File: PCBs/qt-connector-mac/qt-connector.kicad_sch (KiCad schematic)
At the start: 4 parts, among them K1 Quicktake, K2 Modem port, K3 Printer port, K4 ImageWriter

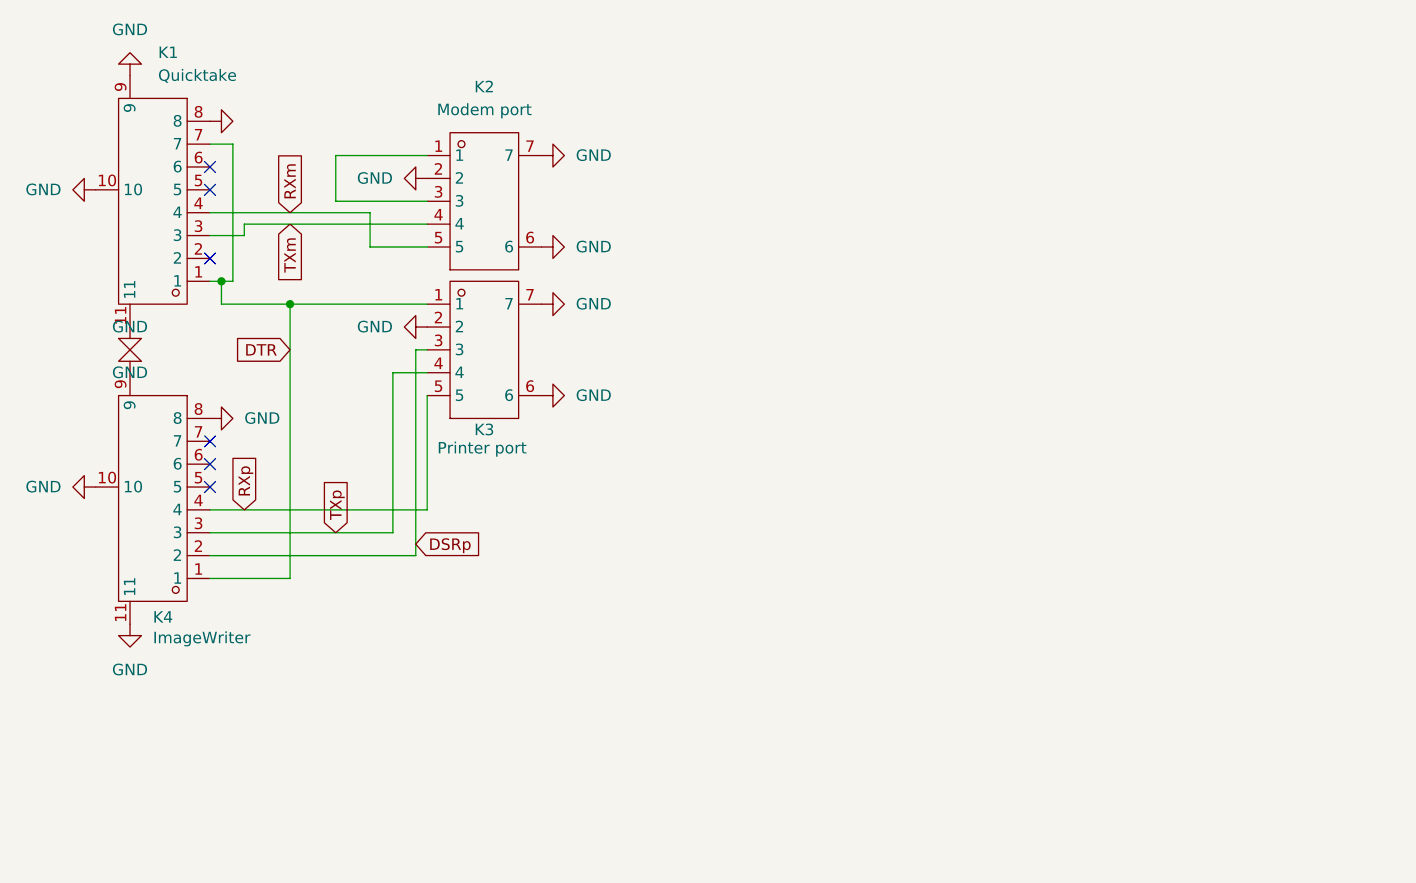
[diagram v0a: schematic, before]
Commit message: Update to new lib
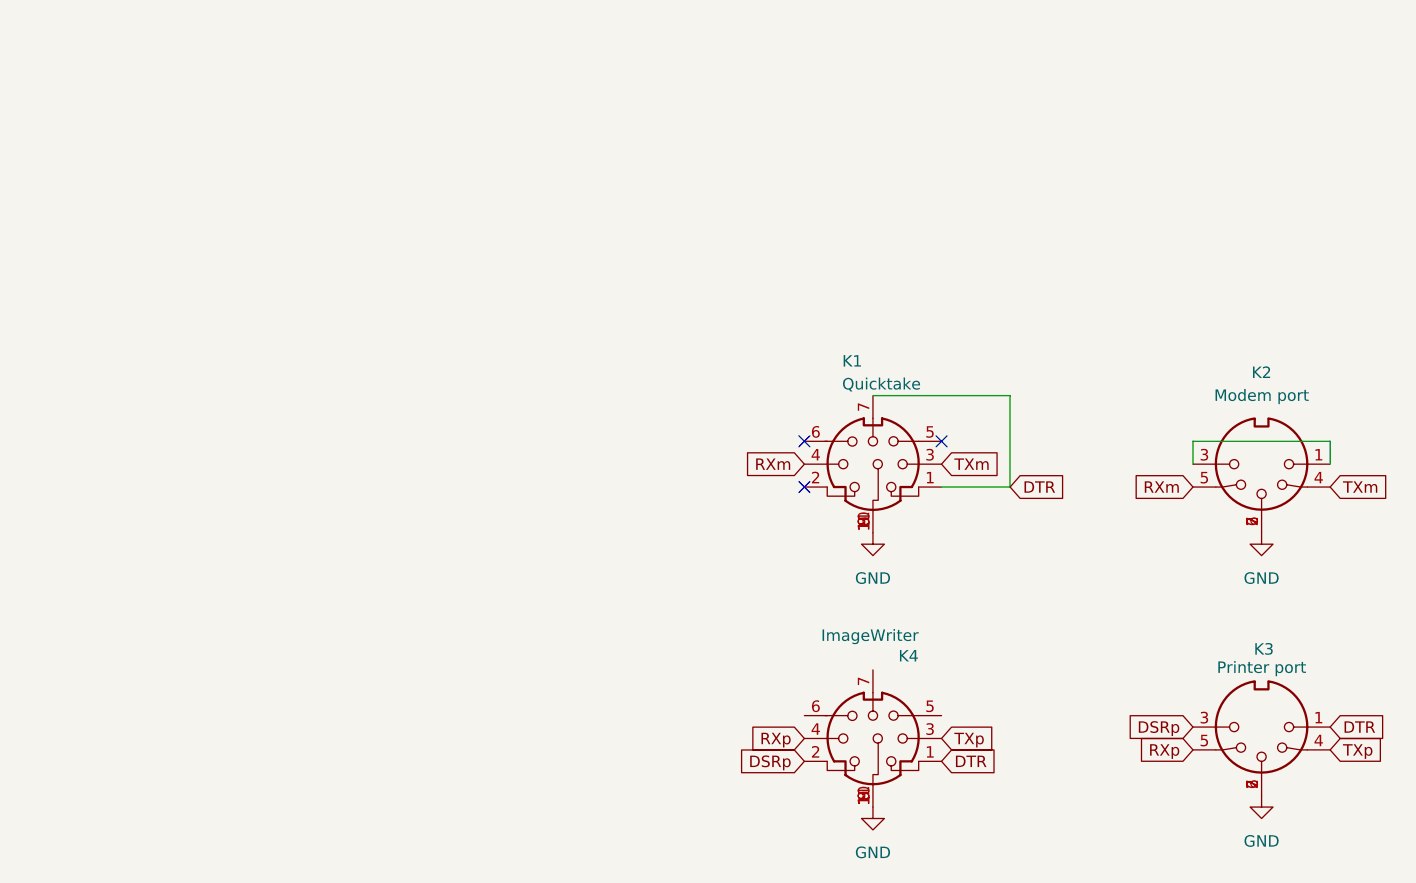
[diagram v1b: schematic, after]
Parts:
- K1, K4: footprint DIN5:MINI-DIN8 -> Colins-Kicad:MINI-DIN8-F C20611694; symbol DIN:DIN-802 -> Colins-Kicad:Serial_Mini-DIN-8
- K2, K3: footprint DIN5:CONN-TH_DIN-504-M10 -> Colins-Kicad:DIN-5-M C23689428; symbol ProLib_pcs_2026-04-19:DIN-504 -> Colins-Kicad:DIN-5_180degree
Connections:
- no-connect marks 6 -> 3
